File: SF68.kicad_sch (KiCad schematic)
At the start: 24 parts, among them J14 pwrjack, SW1 pwrsw, SW2 ressw, U11 68HC000P10, U14 74HC74, U17 74HC04, U22 74HC05, U27 74HC14, X1 CXO_DIP8

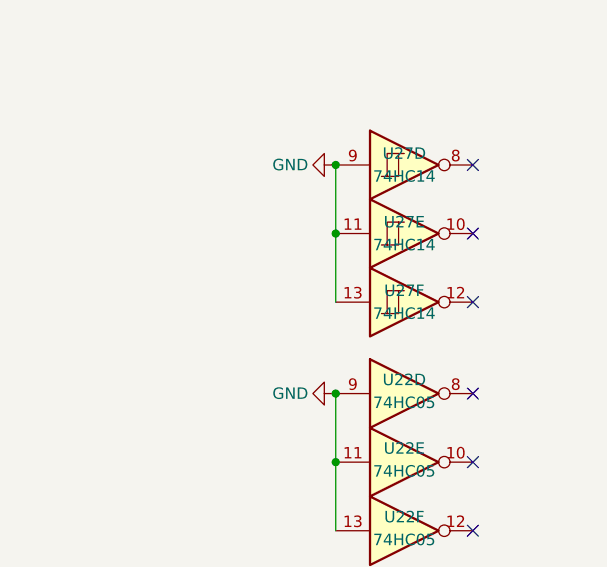
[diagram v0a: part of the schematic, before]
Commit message: applied sf68 & ps2 fixes stash from master
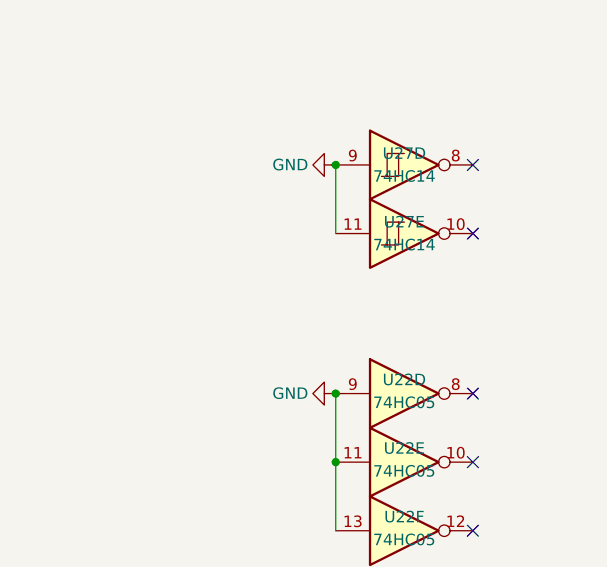
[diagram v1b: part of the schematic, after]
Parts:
- removed unit 6 of U27
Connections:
- no-connect marks 8 -> 7
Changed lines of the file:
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@@
 	)
 	(junction
-		(at 322.58 45.72)
-		(diameter 0)
-		(color 0 0 0 0)
-	)
-	(junction
 		(at 69.85 24.13)
 		(diameter 0)
@@
 		(at 337.82 38.1)
 	)
-	(no_connect
-		(at 337.82 53.34)
-	)
 	(bus_entry
 		(at 181.61 73.66)
@@
 		)
 	)
-	(wire
-		(pts
-			(xy 322.58 45.72) (xy 322.58 53.34)
-		)
-		(stroke
-			(width 0)
-			(type default)
-		)
-	)
 	(bus
 		(pts
@@
 				)
 			)
-		)
-	)
-	(symbol
-		(lib_id "74xx:74HC14")
-		(at 330.2 53.34 0)
-		(unit 6)
-		(exclude_from_sim no)
-		(in_bom yes)
-		(on_board yes)
-		(dnp no)
-		(property "Reference" "U27"
-			(at 330.2 52.07 0)
-			(effects
-				(font
-					(size 1.27 1.27)
-				)
-			)
-		)
-		(property "Value" "74HC14"
-			(at 330.2 54.61 0)
-			(effects
-				(font
-					(size 1.27 1.27)
-				)
-			)
-		)
-		(property "Footprint" "Package_DIP:DIP-14_W7.62mm"
-			(at 330.2 53.34 0)
-			(effects
-				(font
-					(size 1.27 1.27)
-				)
-				(hide yes)
-			)
-		)
-		(property "Datasheet" ""
-			(at 330.2 53.34 0)
-			(effects
-				(font
-					(size 1.27 1.27)
-				)
-				(hide yes)
-			)
-		)
-		(property "Description" ""
-			(at 330.2 53.34 0)
-			(effects
-				(font
-					(size 1.27 1.27)
-				)
-				(hide yes)
-			)
-		)
-		(pin "1"
-		)
-		(pin "5"
-		)
-		(pin "6"
-		)
-		(pin "4"
-		)
-		(pin "2"
-		)
-		(pin "8"
-		)
-		(pin "9"
-		)
-		(pin "3"
-		)
-		(pin "12"
-		)
-		(pin "10"
-		)
-		(pin "7"
-		)
-		(pin "13"
-		)
-		(pin "14"
-		)
-		(pin "11"
-		)
-		(instances
-			(project "SCRM6816"
-				(path "/56448118-82b3-4e1c-bda3-84d63e01a14a"
-					(reference "U27")
-					(unit 6)
-				)
-			)
